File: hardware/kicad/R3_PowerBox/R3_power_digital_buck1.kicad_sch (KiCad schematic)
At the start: 10 parts, among them U1 TPS62132RGTR

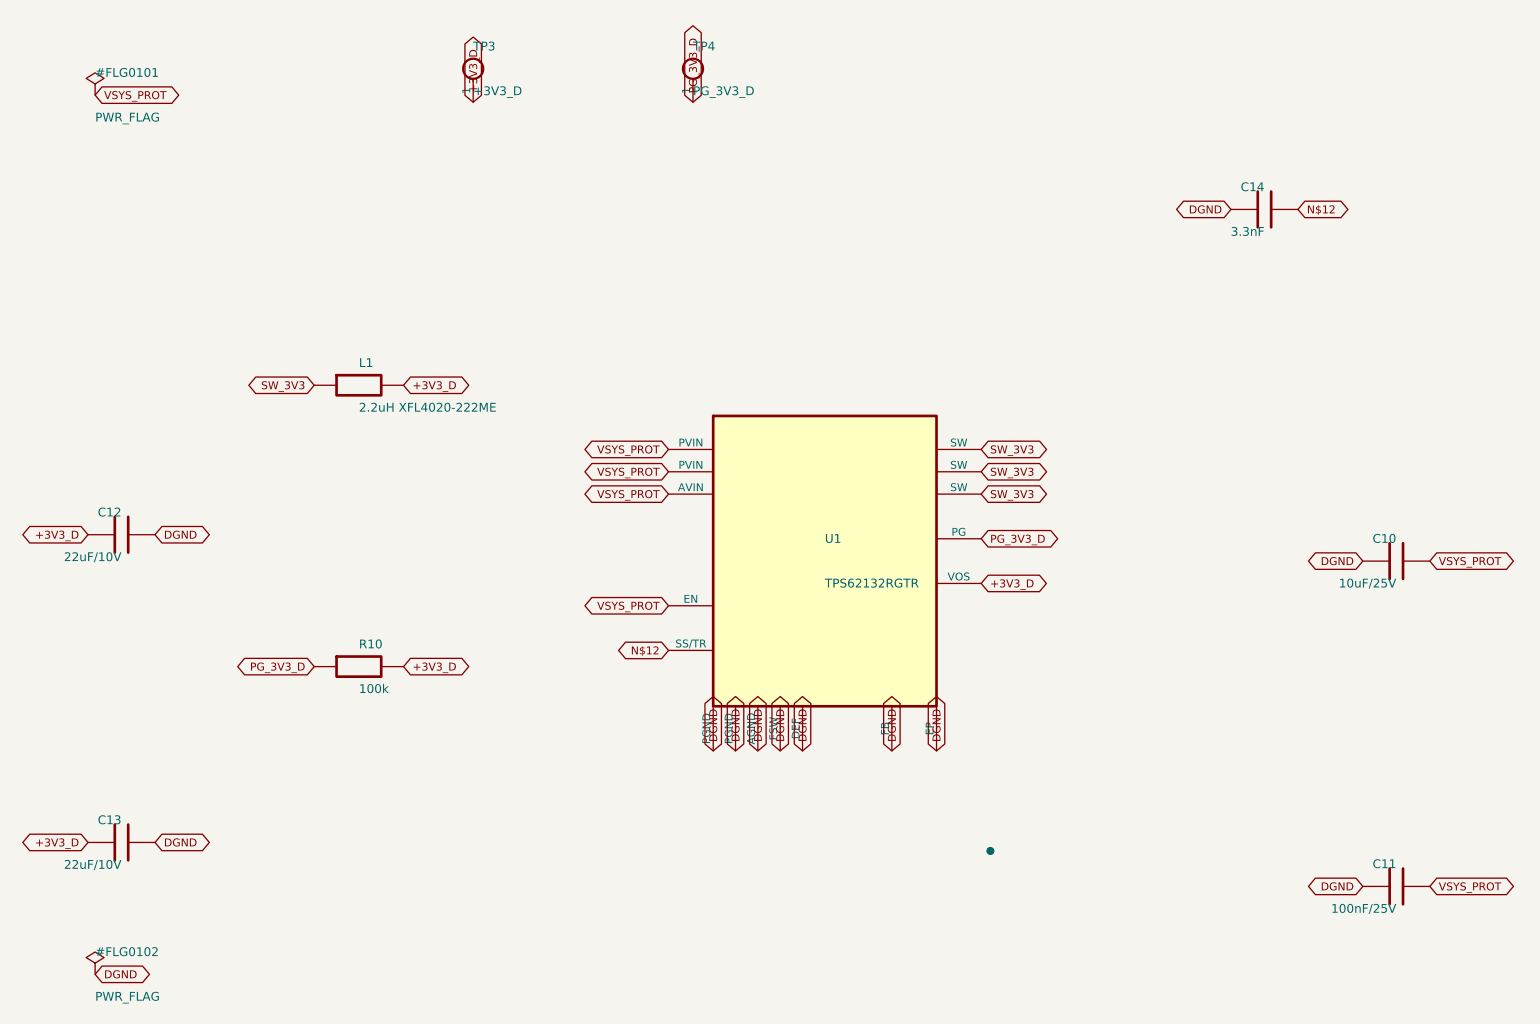
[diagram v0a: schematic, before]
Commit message: Finalize R3 PowerBox pre-placement corrections
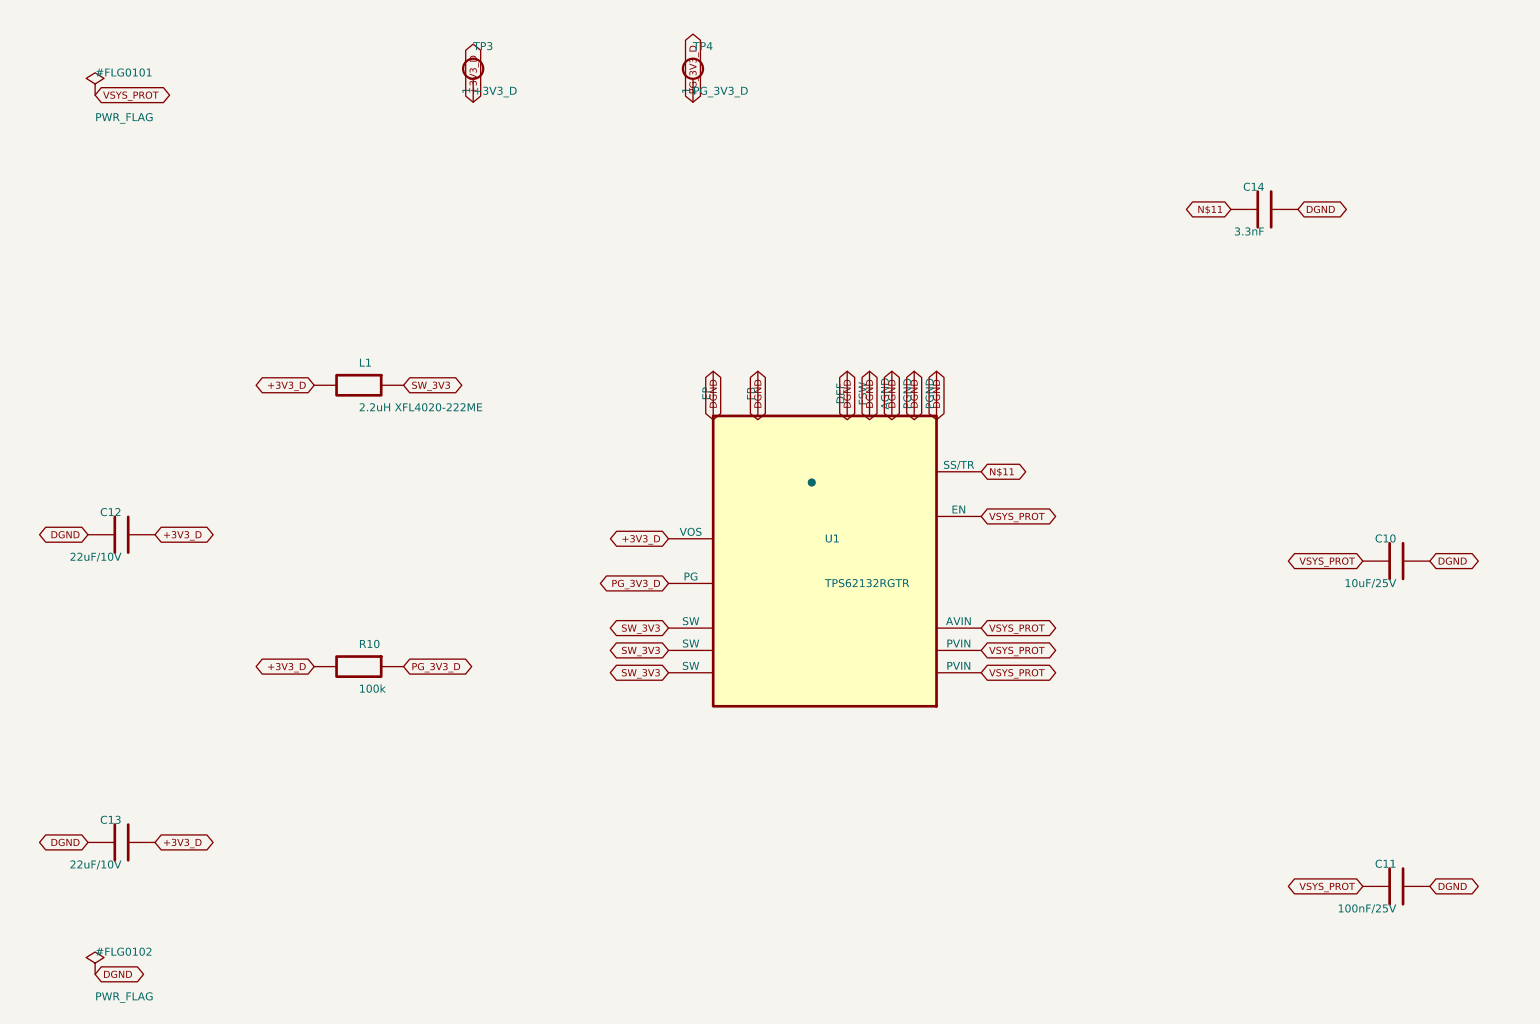
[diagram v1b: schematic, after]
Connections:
- net N$12 renamed N$11
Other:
- moved on the sheet: C10, C11, C12, C13, C14, U1
